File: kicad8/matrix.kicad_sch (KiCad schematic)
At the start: 184 parts, among them SW1 ROT_SKYLOONG_HS

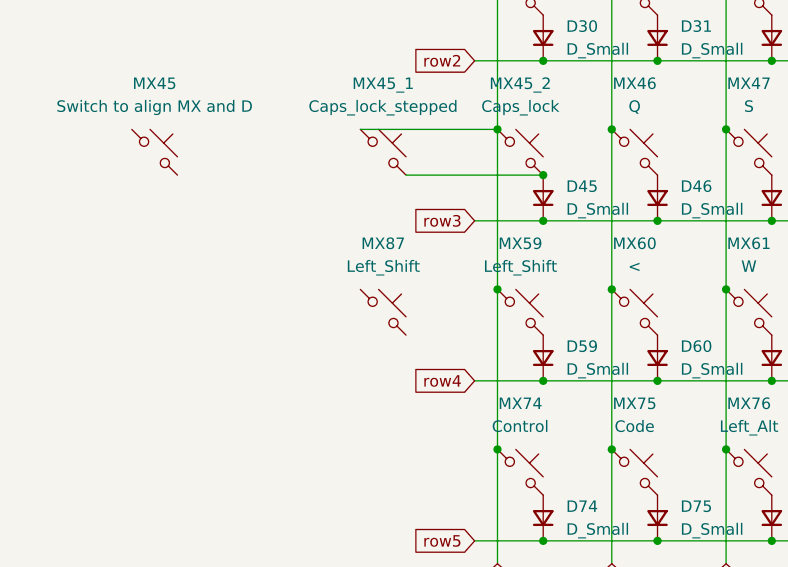
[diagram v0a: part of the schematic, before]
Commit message: Initial branch commit
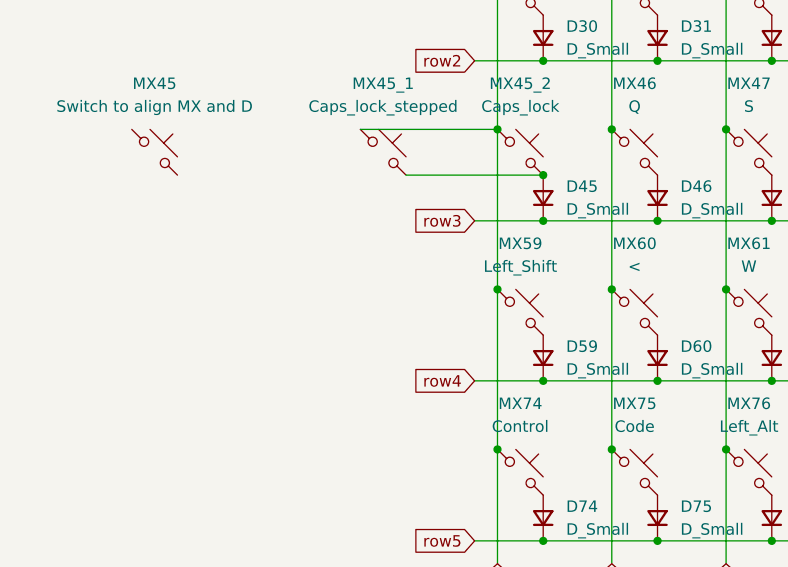
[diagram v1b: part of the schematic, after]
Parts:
- removed MX87: Left_Shift, PCM_marbastlib-mx:SW_MX_HS_CPG151101S11_1u, symbol PCM_marbastlib-mx:MX_SW_HS_CPG151101S11
- R5: footprint Diode_SMD:D_SOD-123 -> Resistor_SMD:R_0402_1005Metric
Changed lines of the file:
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@@
 	)
 	(symbol
-		(lib_id "PCM_marbastlib-mx:MX_SW_HS_CPG151101S11")
-		(at 49.53 96.52 0)
-		(unit 1)
-		(exclude_from_sim no)
-		(in_bom yes)
-		(on_board yes)
-		(dnp no)
-		(fields_autoplaced yes)
-		(property "Reference" "MX87"
-			(at 49.53 88.9 0)
-			(effects
-				(font
-					(size 1.27 1.27)
-				)
-			)
-		)
-		(property "Value" "Left_Shift"
-			(at 49.53 91.44 0)
-			(effects
-				(font
-					(size 1.27 1.27)
-				)
-			)
-		)
-		(property "Footprint" "PCM_marbastlib-mx:SW_MX_HS_CPG151101S11_1u"
-			(at 49.53 96.52 0)
-			(effects
-				(font
-					(size 1.27 1.27)
-				)
-				(hide yes)
-			)
-		)
-		(property "Datasheet" "~"
-			(at 49.53 96.52 0)
-			(effects
-				(font
-					(size 1.27 1.27)
-				)
-				(hide yes)
-			)
-		)
-		(property "Description" "Push button switch, normally open, two pins, 45° tilted, Kailh CPG151101S11 for Cherry MX style switches"
-			(at 49.53 96.52 0)
-			(effects
-				(font
-					(size 1.27 1.27)
-				)
-				(hide yes)
-			)
-		)
-		(pin "1"
-		)
-		(pin "2"
-		)
-		(instances
-			(project "kicad8"
-				(path "/4d291fcf-fdf2-46ba-aa57-60bc75f9cc32/2b97a220-2f1a-429f-8815-0fa3b3b8491d"
-					(reference "MX87")
-					(unit 1)
-				)
-			)
-		)
-	)
-	(symbol
 		(lib_id "Device:D_Small")
 		(at 194.31 66.04 90)
@@
 			)
 		)
-		(property "Footprint" "Diode_SMD:D_SOD-123"
+		(property "Footprint" "Resistor_SMD:R_0402_1005Metric"
 			(at 83.82 151.13 0)
 			(effects
